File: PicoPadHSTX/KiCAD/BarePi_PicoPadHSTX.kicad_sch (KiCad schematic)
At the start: 13 parts, among them IC1 Raspberry Pi Pico 2, J1 OUT, J2 DISPLAY

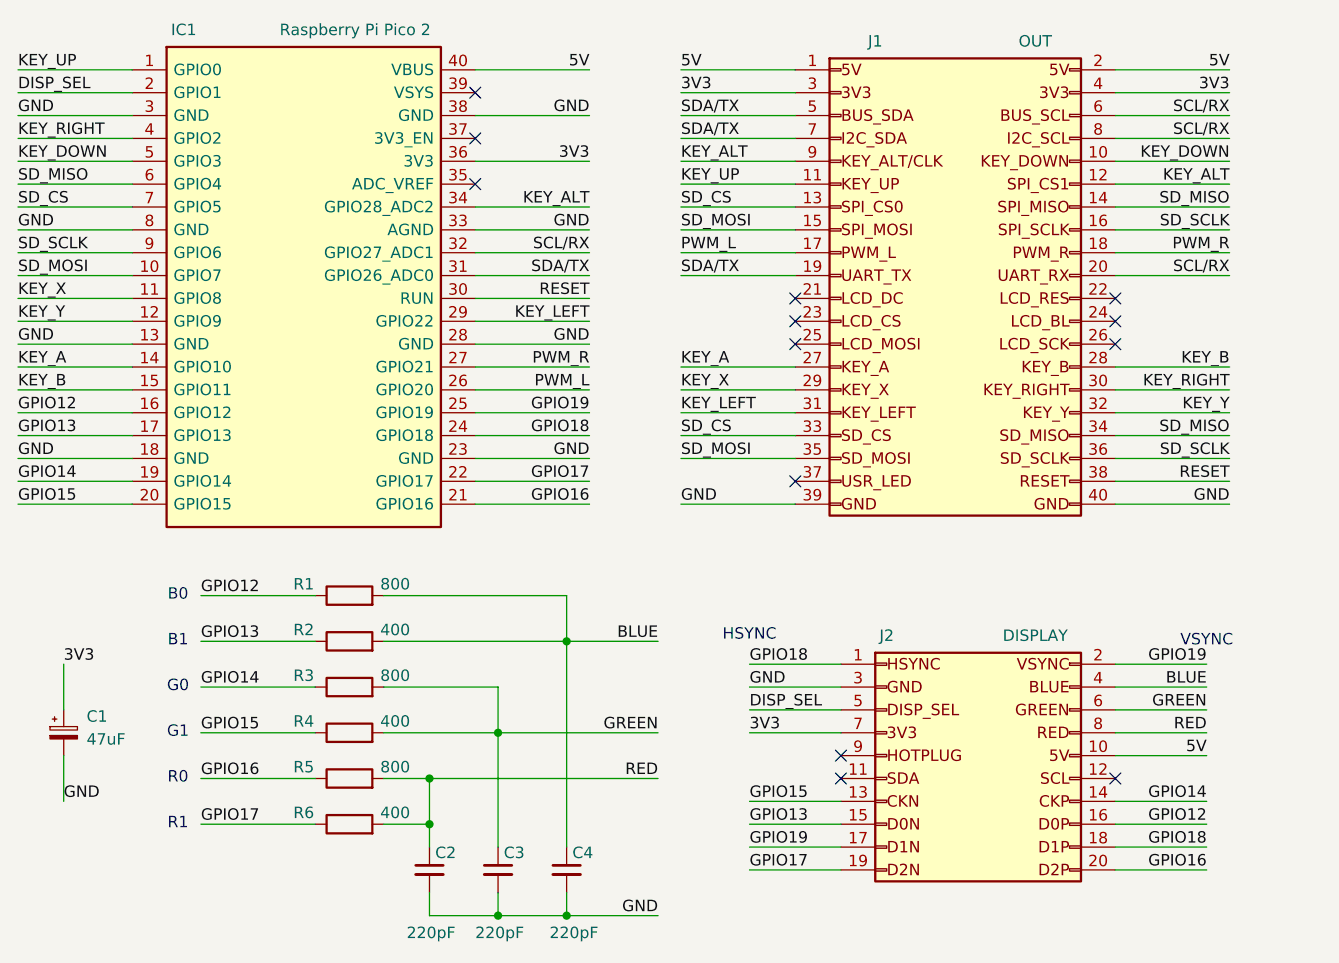
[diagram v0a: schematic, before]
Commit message: init
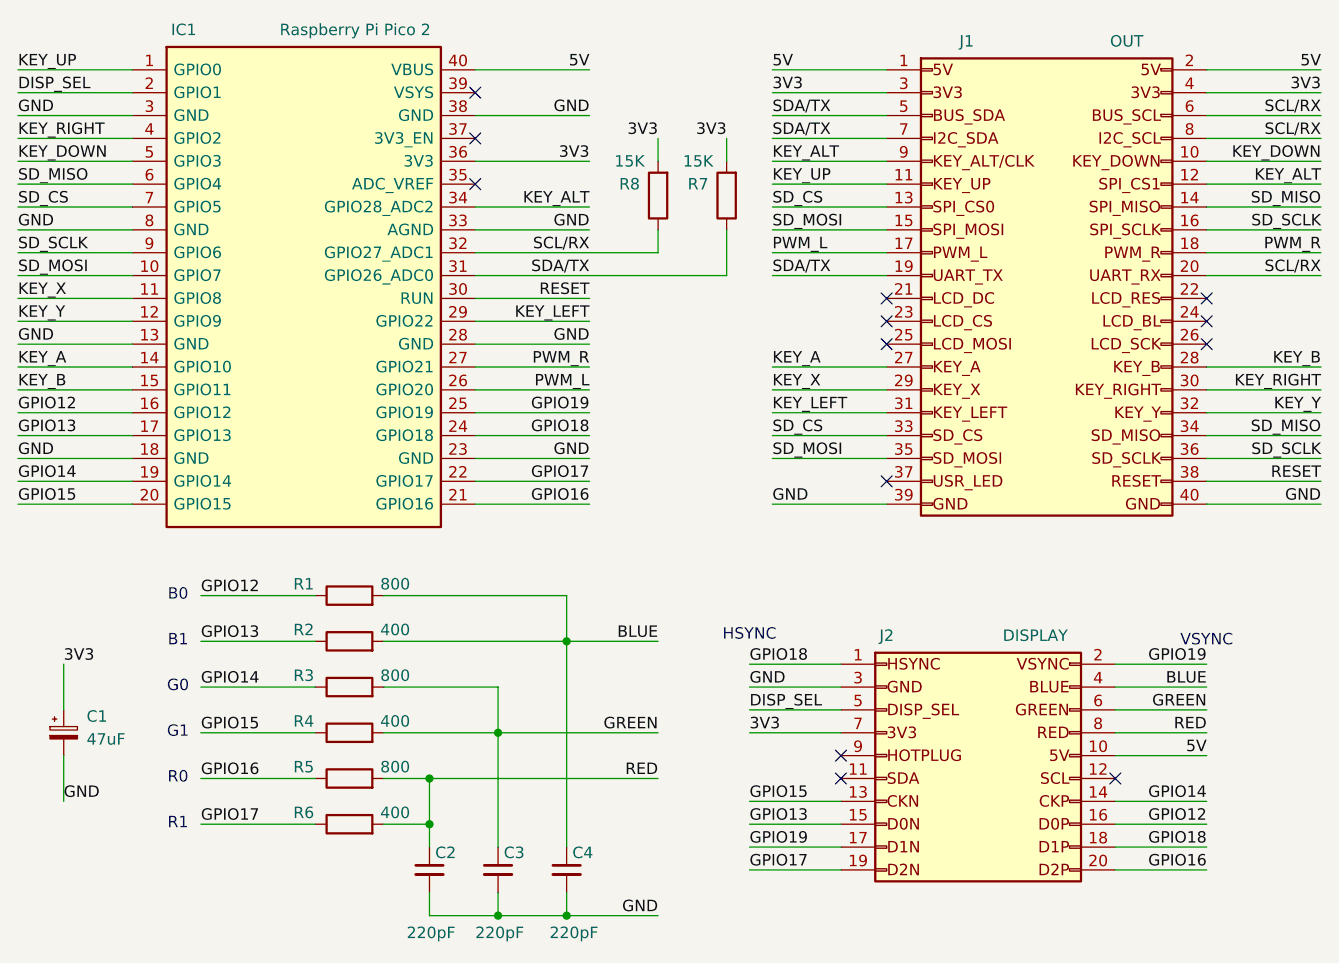
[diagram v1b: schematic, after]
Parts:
- added R7, R8: 15K, Resistor_SMD:R_1206_3216Metric_Pad1.30x1.75mm_HandSolder, symbol Device:R
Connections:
- net 3V3: now also R7.2, R8.2
- net SCL/RX: now also R8.1
- net SDA/TX: now also R7.1
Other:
- moved on the sheet: J1
